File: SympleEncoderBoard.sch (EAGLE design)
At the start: 1 part, among them Y1 CSTCE12M0G55-_R0

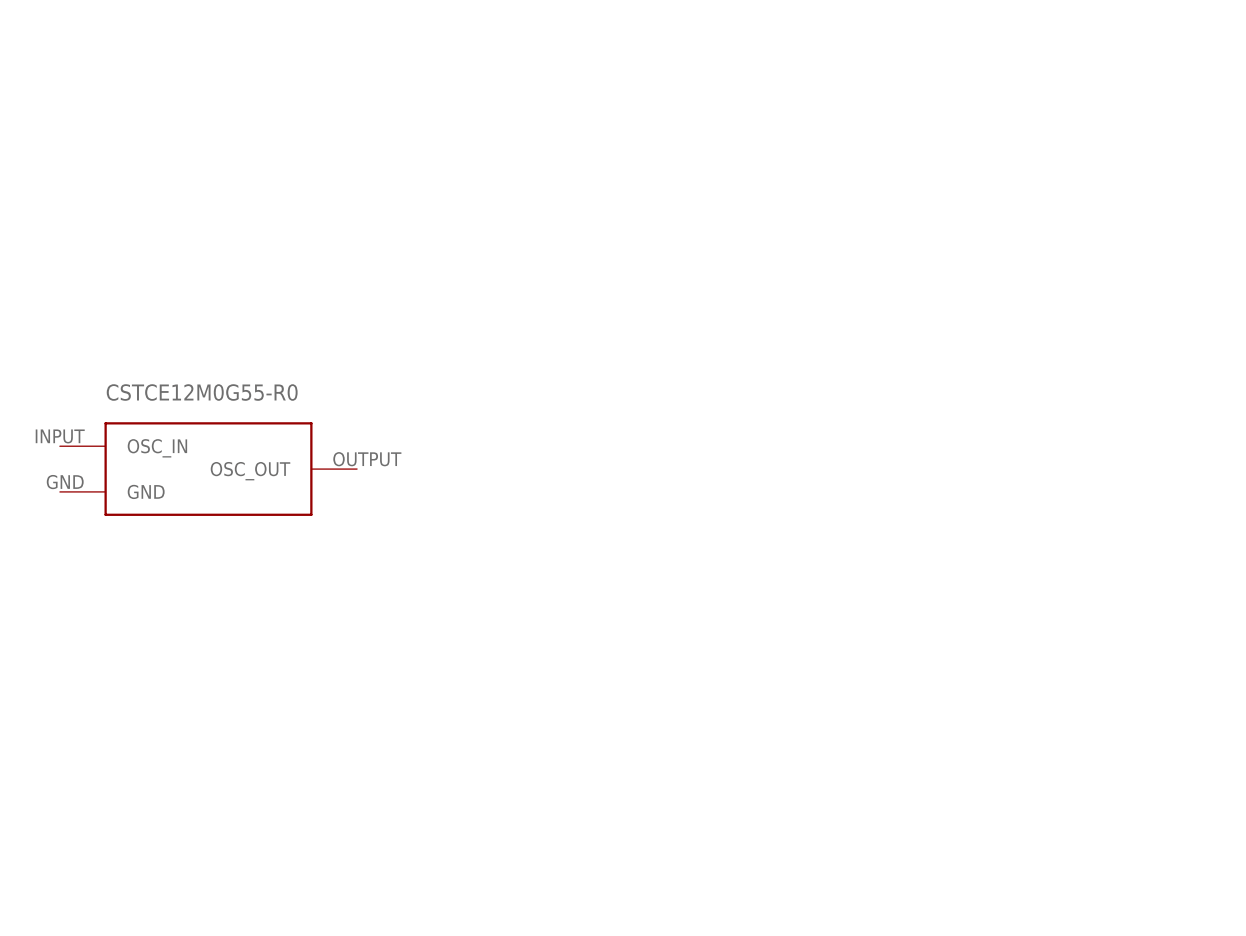
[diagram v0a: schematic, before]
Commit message: ライブラリとかバスを作っただけ
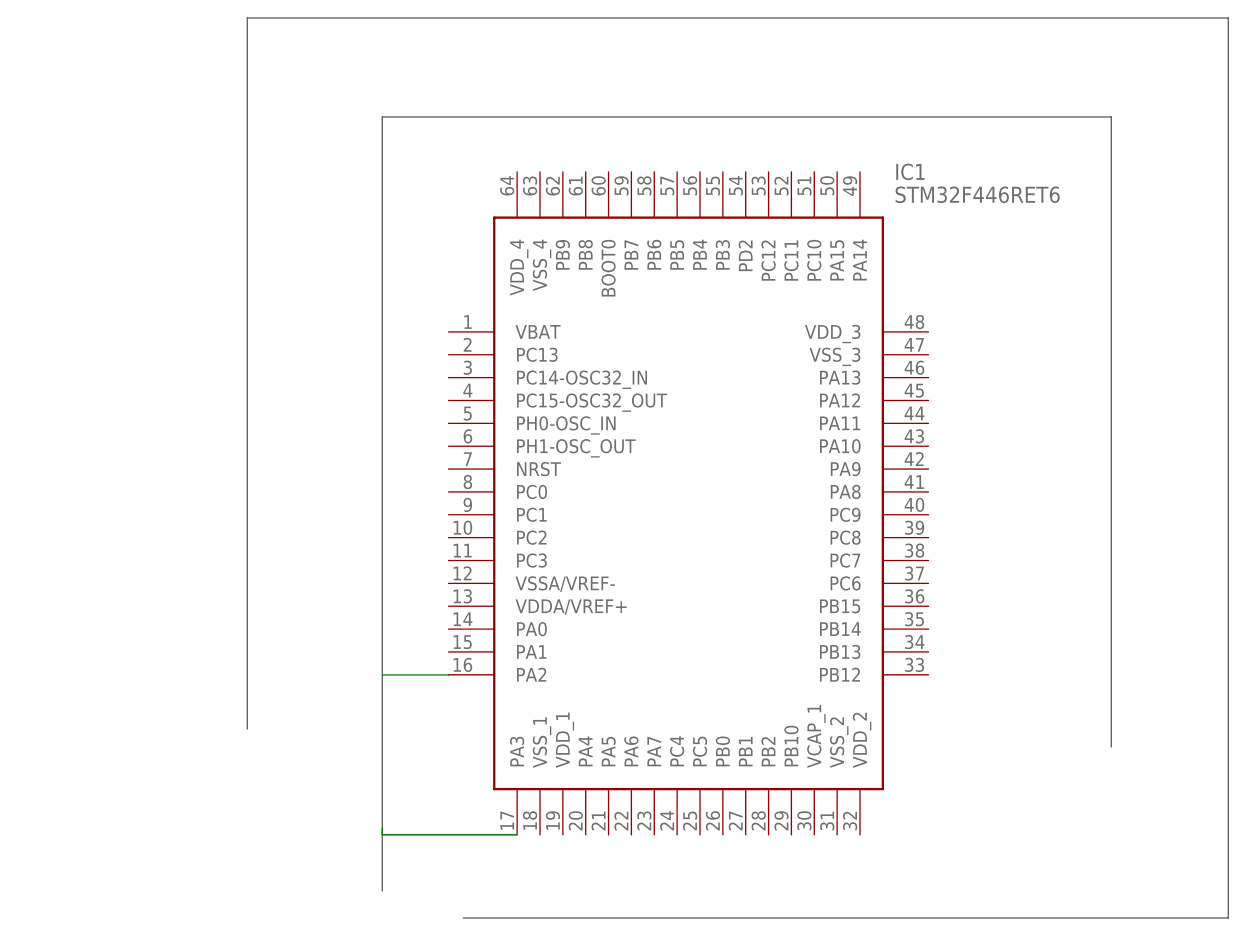
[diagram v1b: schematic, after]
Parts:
- removed Y1: CSTCE12M0G55-_R0, SympleEncoderBoard:CSTCE12M0G55-_R0
- added IC1: STM32F446RET6, STM32F446RET6:STM32F446RET6
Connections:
- new net VCP_RX: IC1.PA3
- new net VCP_TX: IC1.PA2
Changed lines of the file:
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@@
 <setting verticaltext="up"/>
 </settings>
-<grid distance="0.1" unitdist="inch" unit="inch" style="lines" multiple="1" display="no" altdistance="0.01" altunitdist="inch" altunit="inch"/>
+<grid distance="1" unitdist="mm" unit="mm" style="lines" multiple="1" display="yes" altdistance="0.25" altunitdist="mm" altunit="mm"/>
 <layers>
 <layer number="1" name="Top" color="4" fill="1" visible="no" active="no"/>
@@
 </classes>
 <parts>
-<part name="Y1" library="SympleEncoderBoard" deviceset="CSTCE12M0G55-_R0" device=""/>
+<part name="IC1" library="STM32F446RET6" deviceset="STM32F446RET6" device=""/>
 </parts>
 <sheets>
@@
 </plain>
 <instances>
-<instance part="Y1" gate="G$1" x="55.88" y="55.88" smashed="yes"/>
+<instance part="IC1" gate="G$1" x="86.36" y="71.12" smashed="yes">
+<attribute name="NAME" x="135.89" y="88.9" size="1.778" layer="95" align="center-left"/>
+<attribute name="VALUE" x="135.89" y="86.36" size="1.778" layer="96" align="center-left"/>
+</instance>
 </instances>
 <busses>
+<bus name="+3.3V,GND,NRST,SWCLK,SWDIO,SWO,VCP_RX,VCP_TX">
+<segment>
+<wire x1="79" y1="9" x2="79" y2="95" width="0.762" layer="92"/>
+<wire x1="79" y1="95" x2="160" y2="95" width="0.762" layer="92"/>
+<wire x1="160" y1="95" x2="160" y2="25" width="0.762" layer="92"/>
+</segment>
+</bus>
+<bus name="+3.3V,+5V,CAN_RX,CAN_TX,EN1_A,EN1_B,EN2_A,EN2_B,EN3_A,EN3_B,EN4_A,EN4_B,ENX_A,ENX_B,ENY_A,ENY_B,ERRORLED,GND,I2C_SCL,I2C_SDA,LED1,LED2,LEDGYRO,OSC_IN,OSC_OUT,SW1,SW2,SW3,SW4,SW5,SW6,SW7,SW8,SW9">
+<segment>
+<wire x1="173" y1="6" x2="88" y2="6" width="0.762" layer="92"/>
+<wire x1="173" y1="6" x2="173" y2="106" width="0.762" layer="92"/>
+<wire x1="173" y1="106" x2="64" y2="106" width="0.762" layer="92"/>
+<wire x1="64" y1="106" x2="64" y2="27" width="0.762" layer="92"/>
+</segment>
+</bus>
 </busses>
 <nets>
+<net name="VCP_RX" class="0">
+<segment>
+<pinref part="IC1" gate="G$1" pin="PA3"/>
+<wire x1="93.98" y1="15.24" x2="79" y2="15.24" width="0.1524" layer="91"/>
+<wire x1="79" y1="15.24" x2="79" y2="16" width="0.1524" layer="91"/>
+</segment>
+</net>
+<net name="VCP_TX" class="0">
+<segment>
+<pinref part="IC1" gate="G$1" pin="PA2"/>
+<wire x1="86.36" y1="33.02" x2="86.36" y2="33" width="0.1524" layer="91"/>
+<wire x1="86.36" y1="33" x2="79" y2="33" width="0.1524" layer="91"/>
+</segment>
+</net>
 </nets>
 </sheet>
